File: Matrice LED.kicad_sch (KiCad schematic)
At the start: 5 parts, among them J1 Conn_01x03_Socket, J2 USB_B, J3 USB_B, J4 USB_B

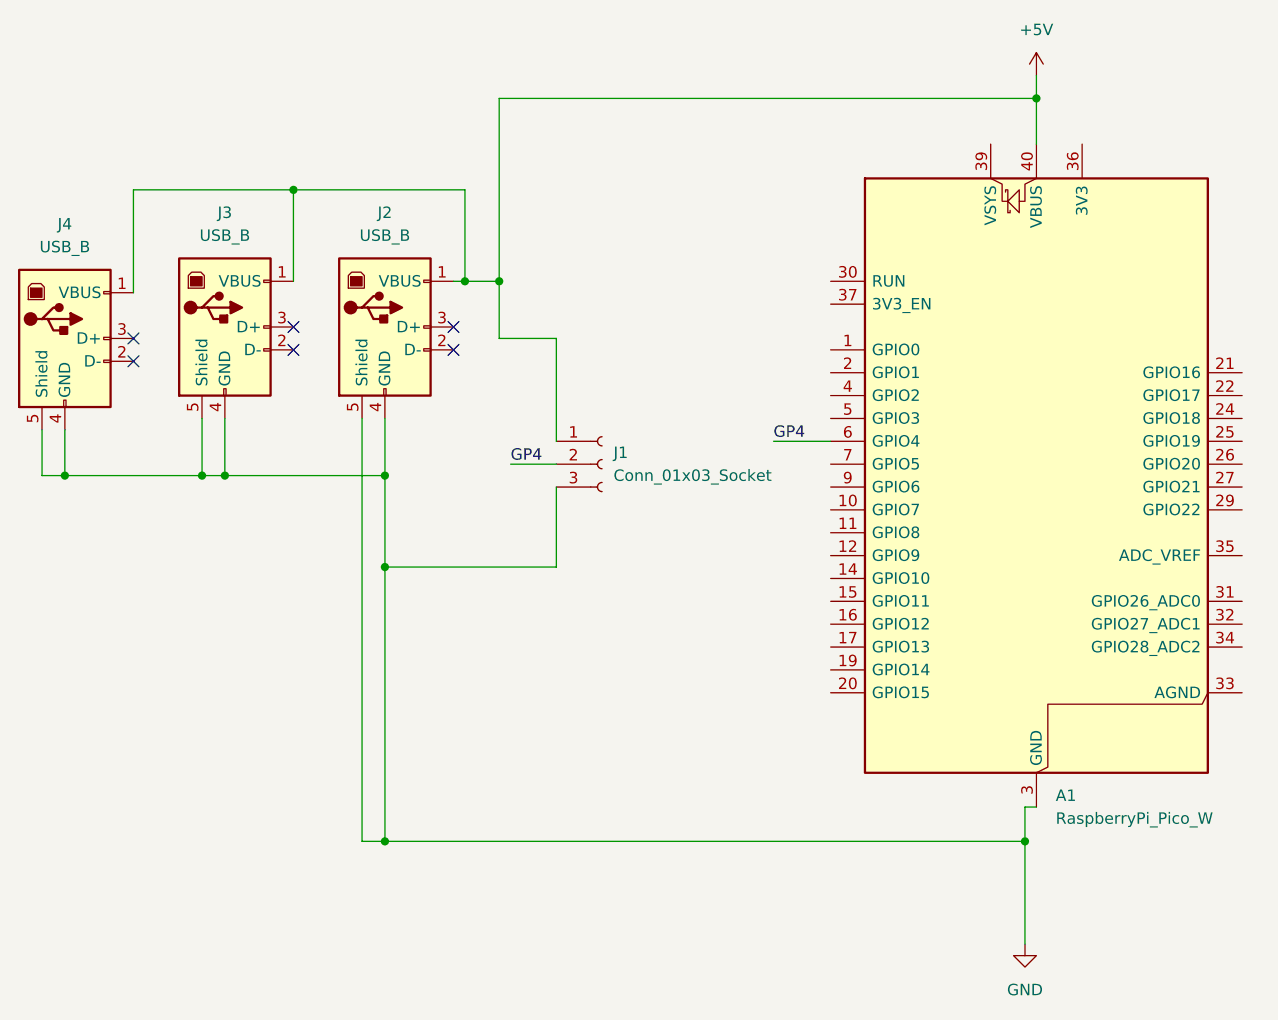
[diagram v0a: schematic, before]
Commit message: Final version
As ordered from PCBWay on 26/03/2026
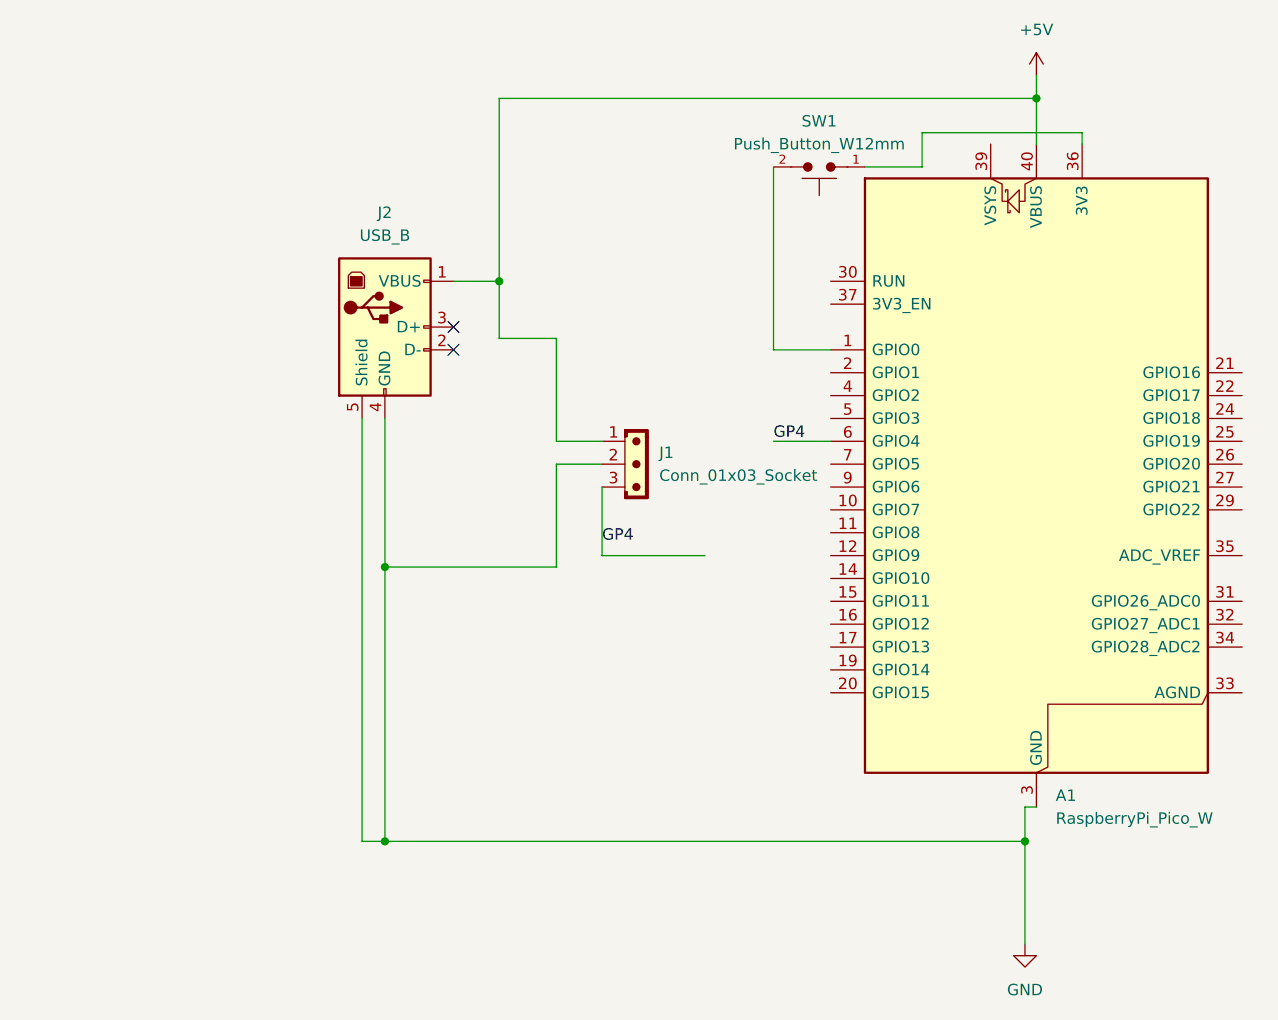
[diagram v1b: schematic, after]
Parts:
- removed J3, J4: USB_B, Connector_USB:USB_B_Lumberg_2411_02_Horizontal, symbol Connector:USB_B
- added SW1: Push_Button_W12mm, PCM_SL_Footprints:Push_Button_W12mm, symbol PCM_SL_Devices:Push_Button_W12mm
- J1: footprint Connector_PinSocket_2.54mm:PinSocket_1x03_P2.54mm_Vertical -> Connector_JST:JST_EH_B3B-EH-A_1x03_P2.50mm_Vertical; symbol Connector:Conn_01x03_Socket -> PCM_SL_Connectors:JST_03
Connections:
- net GND: now also J1.2; no longer J1.3 (Pin_3)
- net GP4: now also J1.3; no longer J1.2 (Pin_2)
- net at A1.1 (GPIO0): now also SW1.2
- net at A1.36 (3V3): now also SW1.1
- no-connect marks 6 -> 2
